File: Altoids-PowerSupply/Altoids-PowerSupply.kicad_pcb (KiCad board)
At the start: 2 copper layers, 90.5 x 56 mm, 0 parts

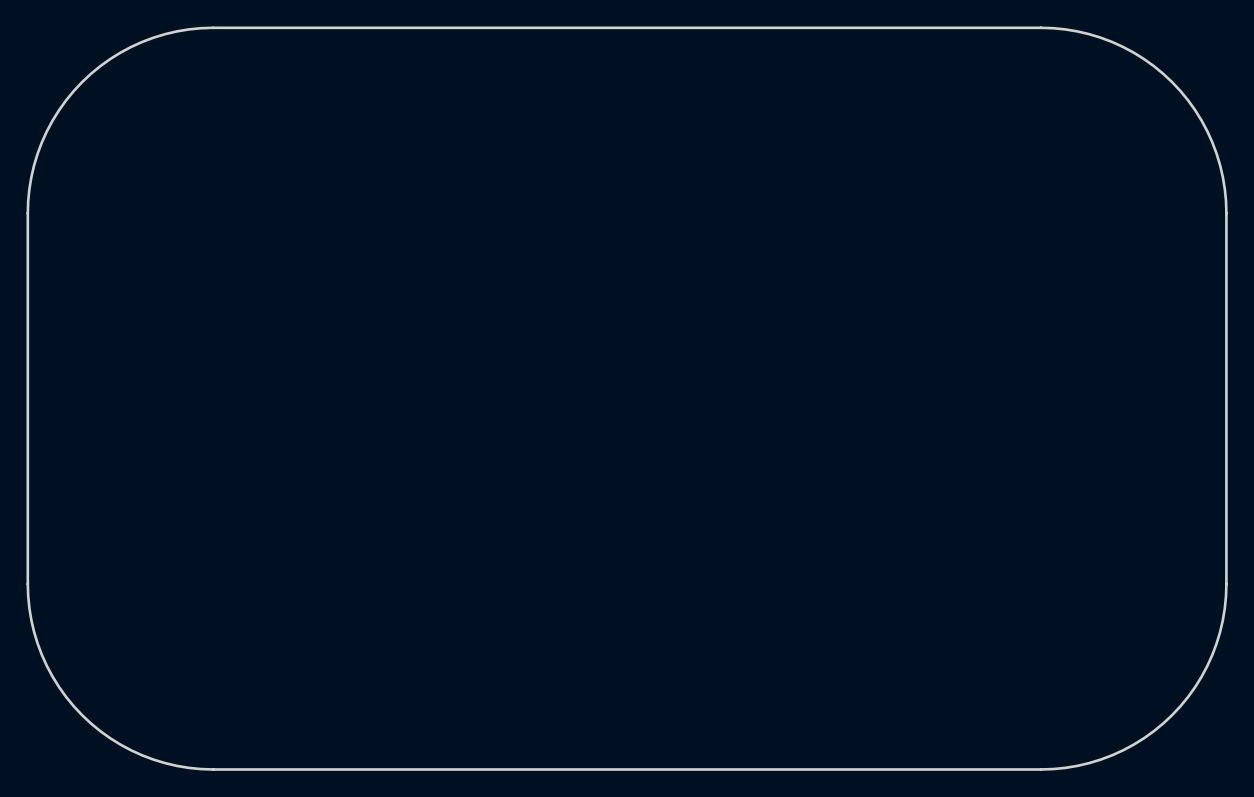
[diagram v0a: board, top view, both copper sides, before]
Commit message: Rev A possibly complete, need to review to ensure no errors. Generated some preliminary gerbers to check things.
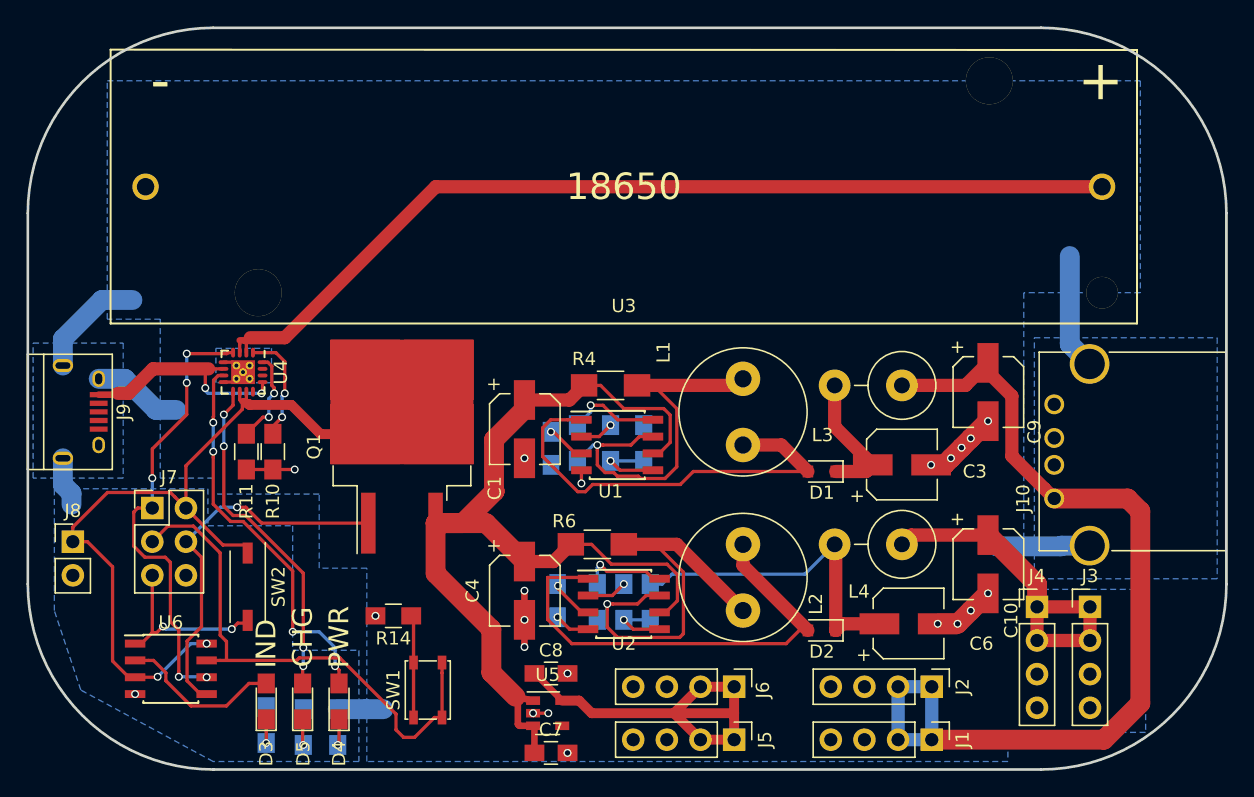
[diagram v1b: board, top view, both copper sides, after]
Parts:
- added C1: 100uF, Capacitors_SMD:CP_Elec_5x5.3, F.Cu at (123.5, 72.3)
- added C10: Cfilter, Capacitors_SMD:CP_Elec_5x5.3, F.Cu at (158.5, 82.5)
- added C2: Ct, Capacitors_SMD:C_0805_HandSoldering, B.Cu at (125.5, 73.8)
- added C3: Co, Capacitors_SMD:CP_Elec_5x5.3, F.Cu at (152.0, 75.0)
- added C4: 100uF, Capacitors_SMD:CP_Elec_5x5.3, F.Cu at (123.5, 84.5)
- added C5: Ct, Capacitors_SMD:C_0805_HandSoldering, B.Cu at (126.0, 85.2)
- added C6: Co, Capacitors_SMD:CP_Elec_5x5.3, F.Cu at (152.5, 87.0)
- added C7: 1uF, Capacitors_SMD:C_0805_HandSoldering, F.Cu at (125.5, 96.8)
- added C8: 1uF, Capacitors_SMD:C_0805_HandSoldering, F.Cu at (125.5, 90.8)
- added C9: Cfilter, Capacitors_SMD:CP_Elec_5x5.3, F.Cu at (158.5, 69.5)
- added D1: 1N5819, Diodes_SMD:D_0805, F.Cu at (145.9, 75.5)
- added D2: 1N5819, Diodes_SMD:D_0805, F.Cu at (145.9, 87.5)
- added D3: LED, LEDs:LED_0805_HandSoldering, F.Cu at (104.0, 92.8)
- added D4: LED, LEDs:LED_0805_HandSoldering, F.Cu at (109.5, 92.8)
- added D5: LED, LEDs:LED_0805_HandSoldering, F.Cu at (106.8, 92.8)
- added J1: Conn_01x04_Male, Pin_Headers:Pin_Header_Straight_1x04_Pitch2.54mm, F.Cu at (154.2, 95.8)
- added J10: USB_A, Connectors:USB_A, F.Cu at (163.5, 77.5)
- added J2: Conn_01x04_Female, Socket_Strips:Socket_Strip_Straight_1x04_Pitch2.54mm, F.Cu at (154.2, 91.8)
- added J3: Conn_01x04_Male, Pin_Headers:Pin_Header_Straight_1x04_Pitch2.54mm, F.Cu at (166.2, 85.7)
- added J4: Conn_01x04_Female, Socket_Strips:Socket_Strip_Straight_1x04_Pitch2.54mm, F.Cu at (162.2, 85.7)
- added J5: Conn_01x04_Male, Pin_Headers:Pin_Header_Straight_1x04_Pitch2.54mm, F.Cu at (139.3, 95.8)
- added J6: Conn_01x04_Female, Socket_Strips:Socket_Strip_Straight_1x04_Pitch2.54mm, F.Cu at (139.3, 91.8)
- added J7: Conn_01x06, Pin_Headers:Pin_Header_Straight_2x03_Pitch2.54mm, F.Cu at (95.4, 78.3)
- added J8: Conn_01x02, Pin_Headers:Pin_Header_Straight_1x02_Pitch2.54mm, F.Cu at (89.4, 80.8)
- added J9: USB_OTG, Connectors:USB_Micro-B, F.Cu at (90.0, 71.0)
- added L1: L, Inductors_THT:L_Radial_D9.5mm_P5.00mm_Fastron_07HVP, F.Cu at (140.0, 73.5)
- added L2: L, Inductors_THT:L_Radial_D9.5mm_P5.00mm_Fastron_07HVP, F.Cu at (140.0, 81.0)
- added L3: 1uH, Inductors_THT:L_Axial_L12.0mm_D5.0mm_P5.08mm_Vertical_Fastron_MISC, F.Cu at (152.0, 69.0)
- added L4: 1uH, Inductors_THT:L_Axial_L12.0mm_D5.0mm_P5.08mm_Vertical_Fastron_MISC, F.Cu at (152.0, 81.0)
- added Q1: Q_PMOS_GDS, TO_SOT_Packages_SMD:TO-263-2, F.Cu at (114.2, 73.6)
- added R1: R1, Resistors_SMD:R_0805_HandSoldering, B.Cu at (130.0, 73.3)
- added R10: 10K, Resistors_SMD:R_0805_HandSoldering, F.Cu at (104.5, 74.0)
- added R11: ISET, Resistors_SMD:R_0805_HandSoldering, F.Cu at (102.5, 74.0)
- added R12: 499, Resistors_SMD:R_0805_HandSoldering, B.Cu at (109.4, 94.8)
- added R13: 499, Resistors_SMD:R_0805_HandSoldering, B.Cu at (106.8, 94.8)
- added R14: 10K, Resistors_SMD:R_0805_HandSoldering, F.Cu at (113.6, 86.4)
- added R2: R2, Resistors_SMD:R_0805_HandSoldering, B.Cu at (132.5, 73.3)
- added R3: 180, Resistors_SMD:R_0805_HandSoldering, B.Cu at (127.5, 73.3)
- added R4: Rsc, Resistors_SMD:R_1206_HandSoldering, F.Cu at (130.0, 69.0)
- added R5: 180, Resistors_SMD:R_0805_HandSoldering, B.Cu at (129.0, 85.3)
- added R6: Rsc, Resistors_SMD:R_1206_HandSoldering, F.Cu at (129.0, 81.0)
- added R7: R2, Resistors_SMD:R_0805_HandSoldering, B.Cu at (133.0, 85.3)
- added R8: R1, Resistors_SMD:R_0805_HandSoldering, B.Cu at (131.0, 85.3)
- added R9: 499, Resistors_SMD:R_0805_HandSoldering, B.Cu at (104.0, 94.7)
- added SW1: SW_Push, Buttons_Switches_SMD:SW_SPST_PTS810, F.Cu at (116.2, 92.0)
- added SW2: SW_DIP_x01, Buttons_Switches_SMD:SW_DIP_x1_W5.08mm_Slide_Copal_CHS-A, F.Cu at (102.6, 84.2)
- added U1: MC34063, Housings_SOIC:SOIC-8_3.9x4.9mm_Pitch1.27mm, F.Cu at (130.5, 73.5)
- added U2: MC34063, Housings_SOIC:SOIC-8_3.9x4.9mm_Pitch1.27mm, F.Cu at (131.0, 85.5)
- added U3: KeyElco-1043P, cust_footprints:KeyElco-1043P, F.Cu at (131.0, 54.0)
- added U4: BQ24230, Housings_DFN_QFN:QFN-16-1EP_3x3mm_Pitch0.5mm_ThermalVias, F.Cu at (102.2, 68.0)
- added U5: AP2127K-3.3TRG1, TO_SOT_Packages_SMD:SOT-23-5, F.Cu at (125.2, 93.8)
- added U6: ATTINY45-20SU, Housings_SOIC:SOIC-8_3.9x4.9mm_Pitch1.27mm, F.Cu at (96.8, 90.4)
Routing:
- net Net-(C1-Pad1): track 0.00 -> 76.6 mm
- net BAT: track 0.00 -> 72.5 mm
- net +5V: track 0.00 -> 70.9 mm
- net Earth: track 0.00 -> 69.2 mm, vias 0 -> 24
- net OUT: track 0.00 -> 58.7 mm, vias 0 -> 2
- net /SCK: track 0.00 -> 40.6 mm
- net Net-(D2-Pad2): track 0.00 -> 35.6 mm
- net Net-(L2-Pad2): track 0.00 -> 34.8 mm, vias 0 -> 1
- net /MISO: track 0.00 -> 34.7 mm, vias 0 -> 5
- net Net-(D1-Pad2): track 0.00 -> 32.8 mm
- net Net-(L1-Pad2): track 0.00 -> 31.1 mm, vias 0 -> 1
- net +3V3: track 0.00 -> 31.1 mm
- net /PGOOD: track 0.00 -> 29.5 mm, vias 0 -> 4
- net Cutoff: track 0.00 -> 28.7 mm, vias 0 -> 1
- net +12V: track 0.00 -> 27.2 mm
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- added copper zone on B.Cu, net Earth
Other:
- board text added: "CHG"
- board text added: "IND"
- board text added: "PWR"
